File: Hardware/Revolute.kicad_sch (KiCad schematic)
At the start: 32 parts, among them J1 USB_A, U1 nRF52840_aQFN73, U2 debug_ports, U3 AP2112K-3.3, X1 32MHZ, X2 32.768 kHz

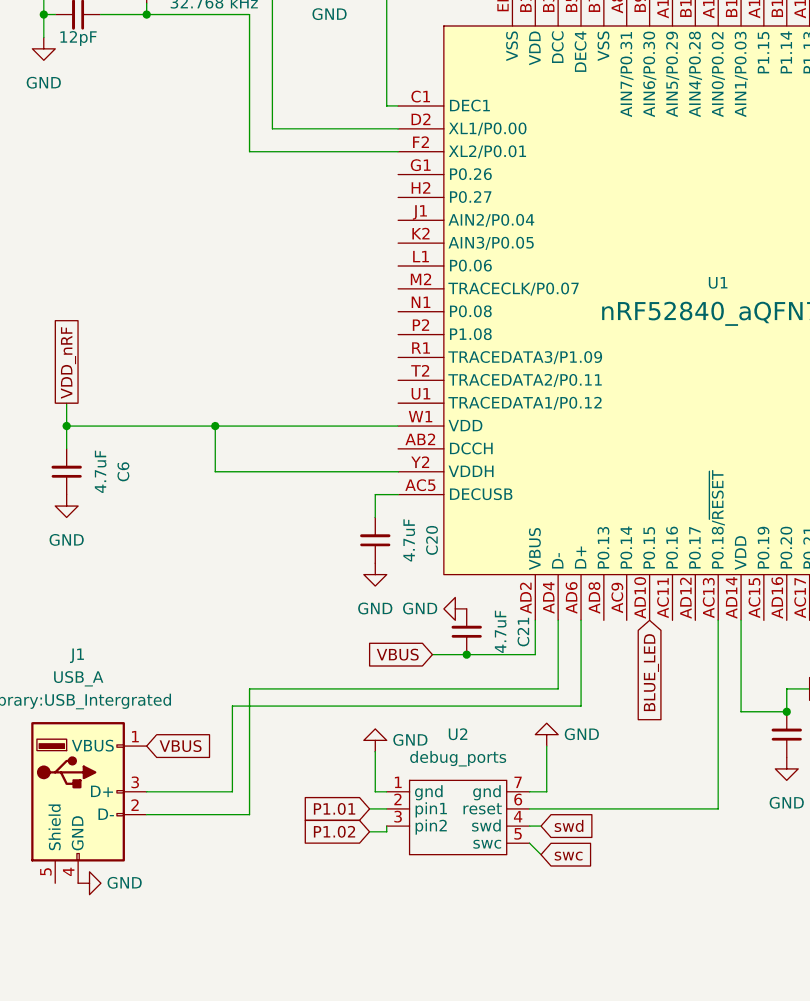
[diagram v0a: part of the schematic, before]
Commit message: version 2 base pcb
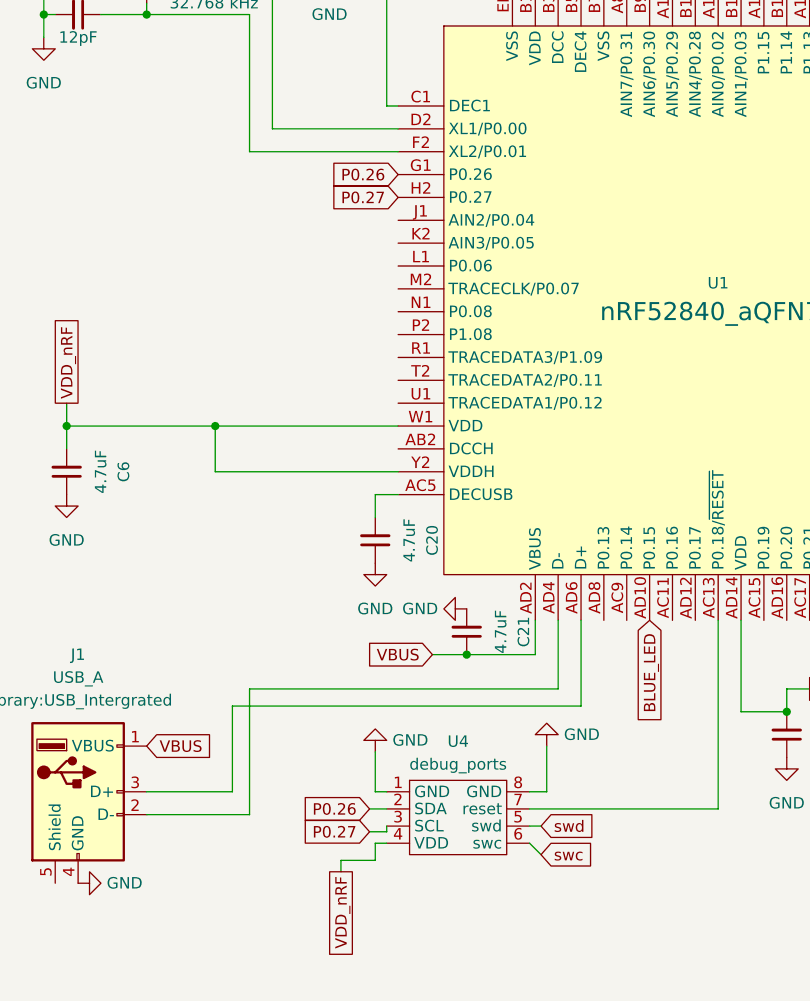
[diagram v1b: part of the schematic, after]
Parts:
- removed U2: debug_ports, Library:Debug pin cluster, symbol New_Library:debug_ports
- added U4: debug_ports, Library:Debug pin cluster, symbol Library:debug_ports
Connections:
- net GND: now also U4.1 (GND), U4.8 (GND)
- net VDD_nRF: now also U4.4 (VDD)
- net swc: now also U4.6 (swc)
- net swd: now also U4.5 (swd)
- net at U1.AC13 (P0.18/~{RESET}): now also U4.7 (reset)
- net P0.26: now reaches U1.G1 (P0.26)
- net P0.26: now also U4.2 (SDA)
- net P0.27: now reaches U1.H2 (P0.27)
- net P0.27: now also U4.3 (SCL)
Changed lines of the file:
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@@
+    (stroke (width 0) (type default))
+  )
+  (wire (pts (xy 114.3 173.355) (xy 113.03 173.355))
     (stroke (width 0) (type default))
   )
@@
   )
   (wire (pts (xy 187.96 90.17) (xy 187.96 64.77))
+    (stroke (width 0) (type default))
+  )
+  (wire (pts (xy 109.22 175.26) (xy 109.22 176.53))
     (stroke (width 0) (type default))
   )
@@
     (stroke (width 0) (type default))
   )
+  (wire (pts (xy 113.03 175.26) (xy 109.22 175.26))
+    (stroke (width 0) (type default))
+  )
   (wire (pts (xy 114.3 91.44) (xy 114.3 71.12))
+    (stroke (width 0) (type default))
+  )
+  (wire (pts (xy 113.03 173.355) (xy 113.03 175.26))
     (stroke (width 0) (type default))
   )
@@
     )
   )
-  (global_label "P1.01" (shape input) (at 112.395 169.545 180) (fields_autoplaced)
-    (effects (font (size 1.27 1.27)) (justify right))
-    (property "Intersheetrefs" "${INTERSHEET_REFS}" (at 104.4786 169.6244 0)
-      (effects (font (size 1.27 1.27)) (justify right) hide)
-    )
-  )
   (global_label "swd" (shape input) (at 186.69 130.81 0) (fields_autoplaced)
     (effects (font (size 1.27 1.27)) (justify left))
@@
     )
   )
+  (global_label "VDD_nRF" (shape passive) (at 109.22 176.53 270) (fields_autoplaced)
+    (effects (font (size 1.27 1.27)) (justify right))
+    (property "Intersheetrefs" "${INTERSHEET_REFS}" (at 109.22 186.4283 90)
+      (effects (font (size 1.27 1.27)) (justify right) hide)
+    )
+  )
   (global_label "P1.01" (shape input) (at 186.69 128.27 0) (fields_autoplaced)
     (effects (font (size 1.27 1.27)) (justify left))
@@
     )
   )
-  (global_label "P1.02" (shape input) (at 112.395 172.085 180) (fields_autoplaced)
-    (effects (font (size 1.27 1.27)) (justify right))
-    (property "Intersheetrefs" "${INTERSHEET_REFS}" (at 104.4786 172.1644 0)
-      (effects (font (size 1.27 1.27)) (justify right) hide)
-    )
-  )
   (global_label "VBUS" (shape input) (at 119.38 152.4 180) (fields_autoplaced)
     (effects (font (size 1.27 1.27)) (justify right))
@@
     )
   )
+  (global_label "P0.26" (shape input) (at 112.395 169.545 180) (fields_autoplaced)
+    (effects (font (size 1.27 1.27)) (justify right))
+    (property "Intersheetrefs" "${INTERSHEET_REFS}" (at 103.9859 169.545 0)
+      (effects (font (size 1.27 1.27)) (justify right) hide)
+    )
+  )
   (global_label "VDD_nRF" (shape passive) (at 78.74 124.46 90) (fields_autoplaced)
     (effects (font (size 1.27 1.27)) (justify left))
@@
     )
   )
+  (global_label "P0.27" (shape input) (at 115.57 101.6 180) (fields_autoplaced)
+    (effects (font (size 1.27 1.27)) (justify right))
+    (property "Intersheetrefs" "${INTERSHEET_REFS}" (at 107.1609 101.6 0)
+      (effects (font (size 1.27 1.27)) (justify right) hide)
+    )
+  )
   (global_label "VDD_nRF" (shape passive) (at 120.65 66.04 90) (fields_autoplaced)
     (effects (font (size 1.27 1.27)) (justify left))
@@
     )
   )
+  (global_label "P0.27" (shape input) (at 112.395 172.085 180) (fields_autoplaced)
+    (effects (font (size 1.27 1.27)) (justify right))
+    (property "Intersheetrefs" "${INTERSHEET_REFS}" (at 103.9859 172.085 0)
+      (effects (font (size 1.27 1.27)) (justify right) hide)
+    )
+  )
   (global_label "VBUS" (shape input) (at 48.895 46.99 180) (fields_autoplaced)
     (effects (font (size 1.27 1.27)) (justify right))
@@
     )
   )
+  (global_label "P0.26" (shape input) (at 115.57 99.06 180) (fields_autoplaced)
+    (effects (font (size 1.27 1.27)) (justify right))
+    (property "Intersheetrefs" "${INTERSHEET_REFS}" (at 107.1609 99.06 0)
+      (effects (font (size 1.27 1.27)) (justify right) hide)
+    )
+  )
   (symbol (lib_id "Device:C_Small") (at 107.95 73.66 0) (unit 1)
     (in_bom yes) (on_board yes) (dnp no)
@@
         (path "/e63e39d7-6ac0-4ffd-8aa3-1841a4541b55"
           (reference "U3") (unit 1)
-        )
-      )
-    )
-  )
-  (symbol (lib_id "New_Library:debug_ports") (at 119.38 167.64 0) (unit 1)
-    (in_bom yes) (on_board yes) (dnp no) (fields_autoplaced)
-    (property "Reference" "U2" (at 122.2375 161.29 0)
-      (effects (font (size 1.27 1.27)))
-    )
-    (property "Value" "debug_ports" (at 122.2375 163.83 0)
-      (effects (font (size 1.27 1.27)))
-    )
-    (property "Footprint" "Library:Debug pin cluster" (at 119.38 167.64 0)
-      (effects (font (size 1.27 1.27)) hide)
-    )
-    (property "Datasheet" "" (at 119.38 167.64 0)
-      (effects (font (size 1.27 1.27)) hide)
-    )
-    (pin "1")
-    (pin "2")
-    (pin "3")
-    (pin "4")
-    (pin "5")
-    (pin "6")
-    (pin "7")
-    (instances
-      (project "Revolute"
-        (path "/e63e39d7-6ac0-4ffd-8aa3-1841a4541b55"
-          (reference "U2") (unit 1)
         )
       )
@@
         )
       )
+    )
+  )
+  (symbol (lib_id "Library:debug_ports") (at 119.38 167.64 0) (unit 1)
+    (in_bom yes) (on_board yes) (dnp no) (fields_autoplaced)
+    (property "Reference" "U4" (at 122.2375 162.052 0)
+      (effects (font (size 1.27 1.27)))
+    )
+    (property "Value" "debug_ports" (at 122.2375 164.592 0)
+      (effects (font (size 1.27 1.27)))
+    )
+    (property "Footprint" "Library:Debug pin cluster" (at 119.38 167.64 0)
+      (effects (font (size 1.27 1.27)) hide)
+    )
+    (property "Datasheet" "" (at 119.38 167.64 0)
+      (effects (font (size 1.27 1.27)) hide)
+    )
+    (pin "1")
+    (pin "2")
+    (pin "3")
+    (pin "4")
+    (pin "5")
+    (pin "6")
+    (pin "7")
+    (pin "8")
+    (instances
+      (project "Revolute"
+        (path "/e63e39d7-6ac0-4ffd-8aa3-1841a4541b55"
+          (reference "U4") (unit 1)
+        )
+      )
